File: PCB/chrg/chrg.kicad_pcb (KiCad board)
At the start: 2 copper layers, 96.5 x 31 mm, 65 parts, among them U1 10k, U11 IP6518, U12 220uF, U13 IP6518, U14 220uF, U15 IP6518, U16 220uF, U17 IP6518, U18 220uF, U2 CH224K

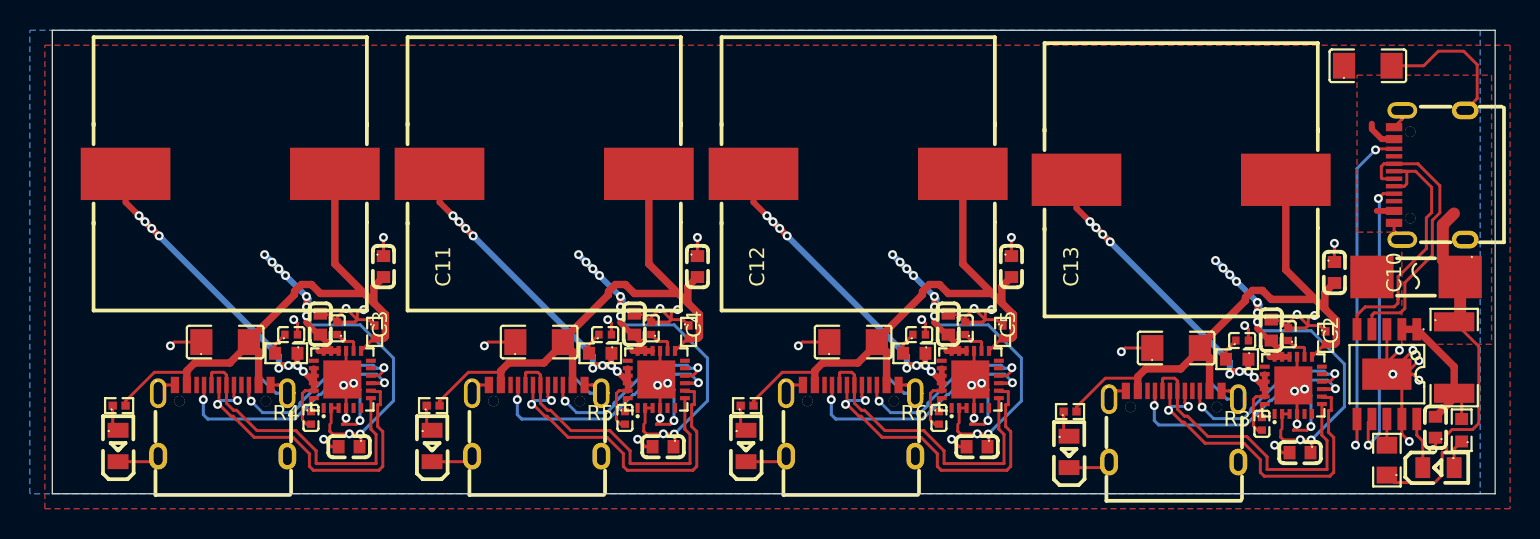
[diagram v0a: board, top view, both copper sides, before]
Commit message: yes
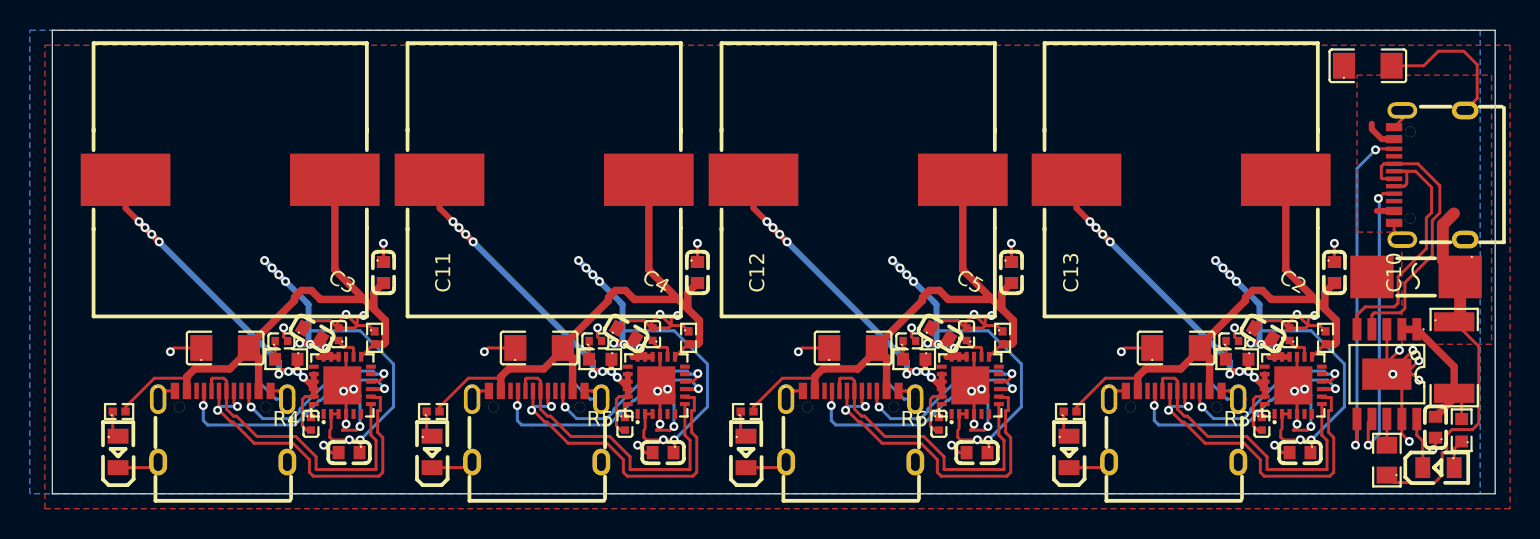
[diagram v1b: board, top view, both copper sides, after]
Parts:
- moved C3 0.83 mm to (41.9, 97.3), turned to -30 degrees
- moved C4 0.83 mm to (62.9, 97.3), turned to -30 degrees
- moved C5 0.83 mm to (83.9, 97.3), turned to -30 degrees
- moved C40 0.78 mm to (39.8, 97.8)
- moved C47 0.78 mm to (60.8, 97.8)
- moved C54 0.78 mm to (81.8, 97.8)
- moved C33 0.66 mm to (103.4, 97.8)
- moved C2 0.59 mm to (105.5, 97.3), turned to -30 degrees
- moved C41 0.40 mm to (43.6, 97.3)
- moved C48 0.40 mm to (64.6, 97.3)
- moved C55 0.40 mm to (85.6, 97.3)
- moved C11 0.40 mm to (46.6, 93.2)
- moved C12 0.40 mm to (67.6, 93.2)
- moved C13 0.40 mm to (88.6, 93.2)
- moved C39 0.40 mm to (41.8, 103.3)
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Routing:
- net VIN: track 126.4 -> 134.8 mm
- net GND: track 150.1 -> 155.1 mm
